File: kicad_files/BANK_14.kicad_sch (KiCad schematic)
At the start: 1 part, among them IC1 XC7S25-1CSGA225C

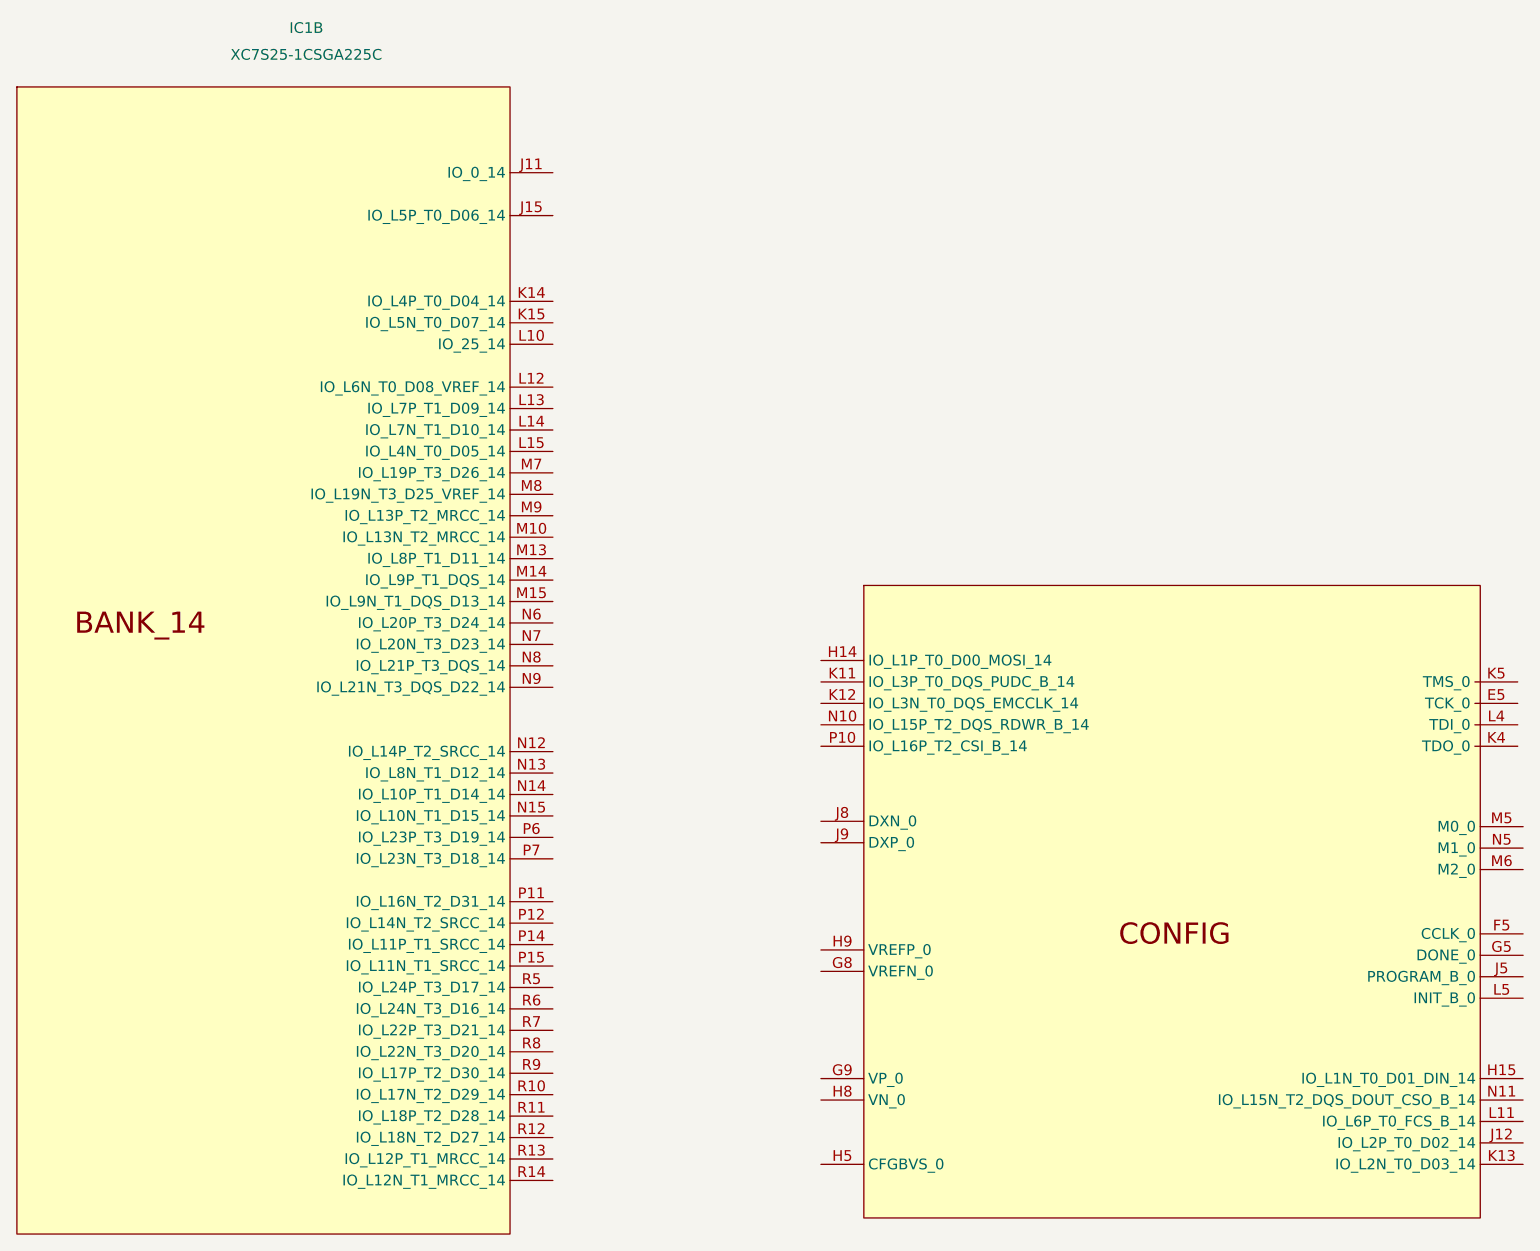
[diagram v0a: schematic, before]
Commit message: schematic updated
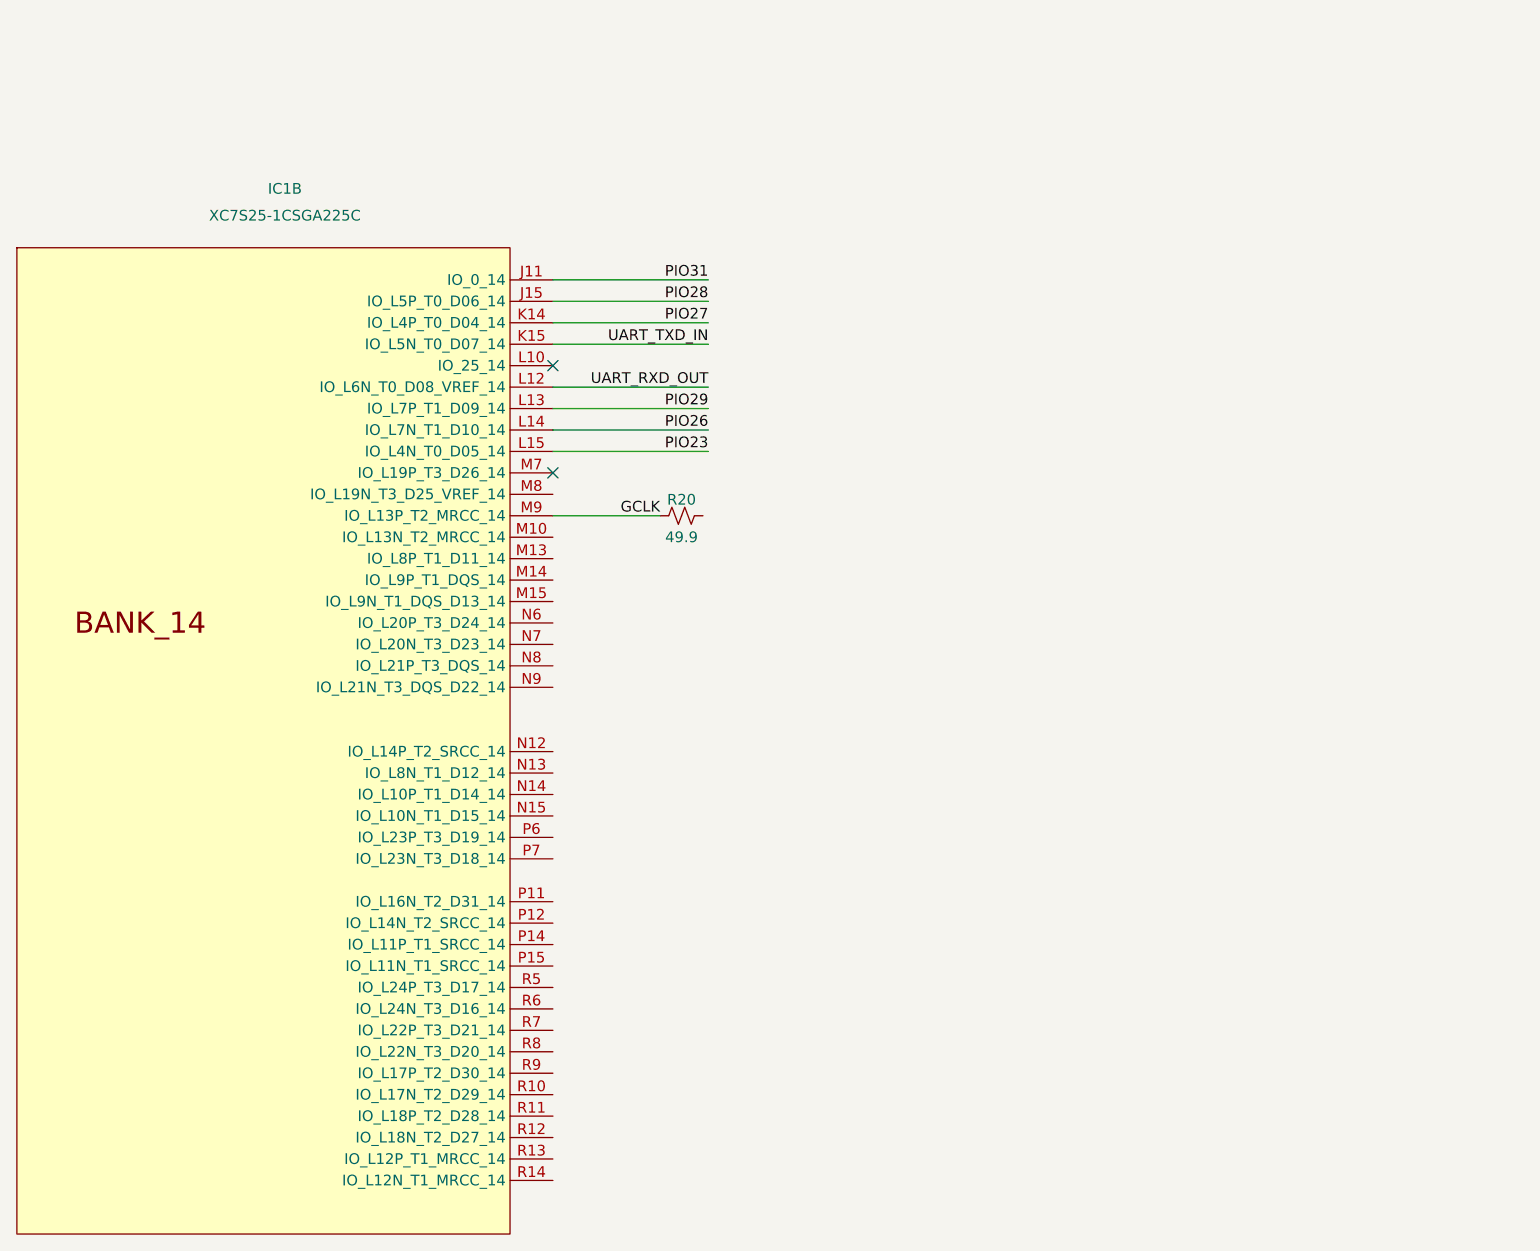
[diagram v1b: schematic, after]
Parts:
- added R20: 49.9, symbol Device:R_Small_US
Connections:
- net PIO31: now reaches IC1.J11 (IO_0_14)
- net PIO28: now reaches IC1.J15 (IO_L5P_T0_D06_14)
- net PIO27: now reaches IC1.K14 (IO_L4P_T0_D04_14)
- net UART_TXD_IN: now reaches IC1.K15 (IO_L5N_T0_D07_14)
- net UART_RXD_OUT: now reaches IC1.L12 (IO_L6N_T0_D08_VREF_14)
- net PIO29: now reaches IC1.L13 (IO_L7P_T1_D09_14)
- net PIO26: now reaches IC1.L14 (IO_L7N_T1_D10_14)
- net PIO23: now reaches IC1.L15 (IO_L4N_T0_D05_14)
- net GCLK: now reaches IC1.M9 (IO_L13P_T2_MRCC_14)
- net GCLK: now also R20.1
- no-connect marks 0 -> 2
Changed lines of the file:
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@@
 (kicad_sch (version 20230121) (generator eeschema)
   (paper "A4")
+  (no_connect (at 132.715 76.835))
+  (no_connect (at 132.715 64.135))
+  (wire (pts (xy 132.715 74.295) (xy 151.13 74.295))
+    (stroke (width 0) (type default))
+  )
+  (wire (pts (xy 132.715 61.595) (xy 151.13 61.595))
+    (stroke (width 0) (type default))
+  )
+  (wire (pts (xy 132.715 71.755) (xy 151.13 71.755))
+    (stroke (width 0) (type default))
+  )
+  (wire (pts (xy 132.715 69.215) (xy 151.13 69.215))
+    (stroke (width 0) (type default))
+  )
+  (wire (pts (xy 132.715 59.055) (xy 151.13 59.055))
+    (stroke (width 0) (type default))
+  )
+  (wire (pts (xy 132.715 56.515) (xy 151.13 56.515))
+    (stroke (width 0) (type default))
+  )
+  (wire (pts (xy 132.715 81.915) (xy 145.415 81.915))
+    (stroke (width 0) (type default))
+  )
+  (wire (pts (xy 132.715 66.675) (xy 151.13 66.675))
+    (stroke (width 0) (type default))
+  )
+  (wire (pts (xy 132.715 53.975) (xy 151.13 53.975))
+    (stroke (width 0) (type default))
+  )
+  (label "PIO29" (at 151.13 69.215 180) (fields_autoplaced)
+    (effects (font (size 1.27 1.27)) (justify right bottom))
+  )
+  (label "PIO23" (at 151.13 74.295 180) (fields_autoplaced)
+    (effects (font (size 1.27 1.27)) (justify right bottom))
+  )
+  (label "GCLK" (at 145.415 81.915 180) (fields_autoplaced)
+    (effects (font (size 1.27 1.27)) (justify right bottom))
+  )
+  (label "PIO27" (at 151.13 59.055 180) (fields_autoplaced)
+    (effects (font (size 1.27 1.27)) (justify right bottom))
+  )
+  (label "UART_RXD_OUT" (at 151.13 66.675 180) (fields_autoplaced)
+    (effects (font (size 1.27 1.27)) (justify right bottom))
+  )
+  (label "UART_TXD_IN" (at 151.13 61.595 180) (fields_autoplaced)
+    (effects (font (size 1.27 1.27)) (justify right bottom))
+  )
+  (label "PIO31" (at 151.13 53.975 180) (fields_autoplaced)
+    (effects (font (size 1.27 1.27)) (justify right bottom))
+  )
+  (label "PIO28" (at 151.13 56.515 180) (fields_autoplaced)
+    (effects (font (size 1.27 1.27)) (justify right bottom))
+  )
+  (label "PIO26" (at 151.13 71.755 180) (fields_autoplaced)
+    (effects (font (size 1.27 1.27)) (justify right bottom))
+  )
   (symbol (lib_id "SamacSys_Parts:XC7S25-1CSGA225C") (at 103.505 100.965 0) (unit 2)
     (in_bom yes) (on_board yes) (dnp no)
-    (property "Reference" "IC1" (at 103.505 24.13 0)
+    (property "Reference" "IC1" (at 100.965 43.18 0)
       (effects (font (size 1.27 1.27)))
     )
-    (property "Value" "XC7S25-1CSGA225C" (at 103.505 27.305 0)
+    (property "Value" "XC7S25-1CSGA225C" (at 100.965 46.355 0)
       (effects (font (size 1.27 1.27)))
     )
@@
     (pin "R1")
     (pin "R15")
-    (pin "E5")
-    (pin "F5")
-    (pin "G5")
-    (pin "G8")
-    (pin "G9")
-    (pin "H14")
-    (pin "H15")
-    (pin "H5")
-    (pin "H8")
-    (pin "H9")
     (pin "J11")
-    (pin "J12")
     (pin "J15")
-    (pin "J5")
-    (pin "J8")
-    (pin "J9")
-    (pin "K11")
-    (pin "K12")
-    (pin "K13")
     (pin "K14")
     (pin "K15")
-    (pin "K4")
-    (pin "K5")
     (pin "L10")
-    (pin "L11")
     (pin "L12")
     (pin "L13")
     (pin "L14")
     (pin "L15")
-    (pin "L4")
-    (pin "L5")
     (pin "M10")
     (pin "M13")
     (pin "M14")
     (pin "M15")
-    (pin "M5")
-    (pin "M6")
     (pin "M7")
     (pin "M8")
     (pin "M9")
-    (pin "N10")
-    (pin "N11")
     (pin "N12")
     (pin "N13")
     (pin "N14")
     (pin "N15")
-    (pin "N5")
     (pin "N6")
     (pin "N7")
     (pin "N8")
     (pin "N9")
-    (pin "P10")
     (pin "P11")
     (pin "P12")
@@
           (reference "IC1") (unit 2)
         )
+        (path "/94bd3a84-5526-4cf2-a5cc-3887356f447c/30d52c37-ae5c-405e-8a78-89b18a6efc4e/af489dd5-0e9e-4b3e-a401-f1288bd8b210"
+          (reference "IC1") (unit 2)
+        )
       )
+    )
+  )
+  (symbol (lib_id "Device:R_Small_US") (at 147.955 81.915 90) (unit 1)
+    (in_bom yes) (on_board yes) (dnp no)
+    (property "Reference" "R20" (at 147.955 80.01 90)
+      (effects (font (size 1.27 1.27)))
+    )
+    (property "Value" "49.9" (at 147.955 84.455 90)
+      (effects (font (size 1.27 1.27)))
+    )
+    (property "Footprint" "" (at 147.955 81.915 0)
+      (effects (font (size 1.27 1.27)) hide)
+    )
+    (property "Datasheet" "~" (at 147.955 81.915 0)
+      (effects (font (size 1.27 1.27)) hide)
+    )
+    (pin "1")
+    (pin "2")
+    (instances
+      (project "sparton_7"
+        (path "/94bd3a84-5526-4cf2-a5cc-3887356f447c/30d52c37-ae5c-405e-8a78-89b18a6efc4e/b9c5b3c3-3c31-4d87-a13a-ee1ac9be93fb"
+          (reference "R20") (unit 1)
+        )
+      )
